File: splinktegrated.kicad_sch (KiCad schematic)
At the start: 65 parts, among them J1 USB_C_Receptacle_USB2.0, J10 NA_Ribbon, J11 NA_Serial, J12 NA_Conn_01x04_Female, J13 Conn_01x01_Socket, J14 Cirque, J15 Conn_01x01_Socket, J16 Conn_01x01_Socket, J17 Conn_01x01_Socket, J2 NA_Conn_01x04_Female, J3 NA_Conn_01x04_Female, J4 NA_Conn_01x04_Female, J5 Conn_01x02, J6 Cirque, J7 NA_trackball, J8 NA_Ribbon, J9 NA_RGB, SW1 NA_SW_SPST, SW2 NA_SW_SPST, U1 RP2040, U2 USBLC6-2P6, U3 XC6210B332MR-G, U4 USBLC6-2P6, U5 W25Q128JVS, Y1 Crystal_GND24

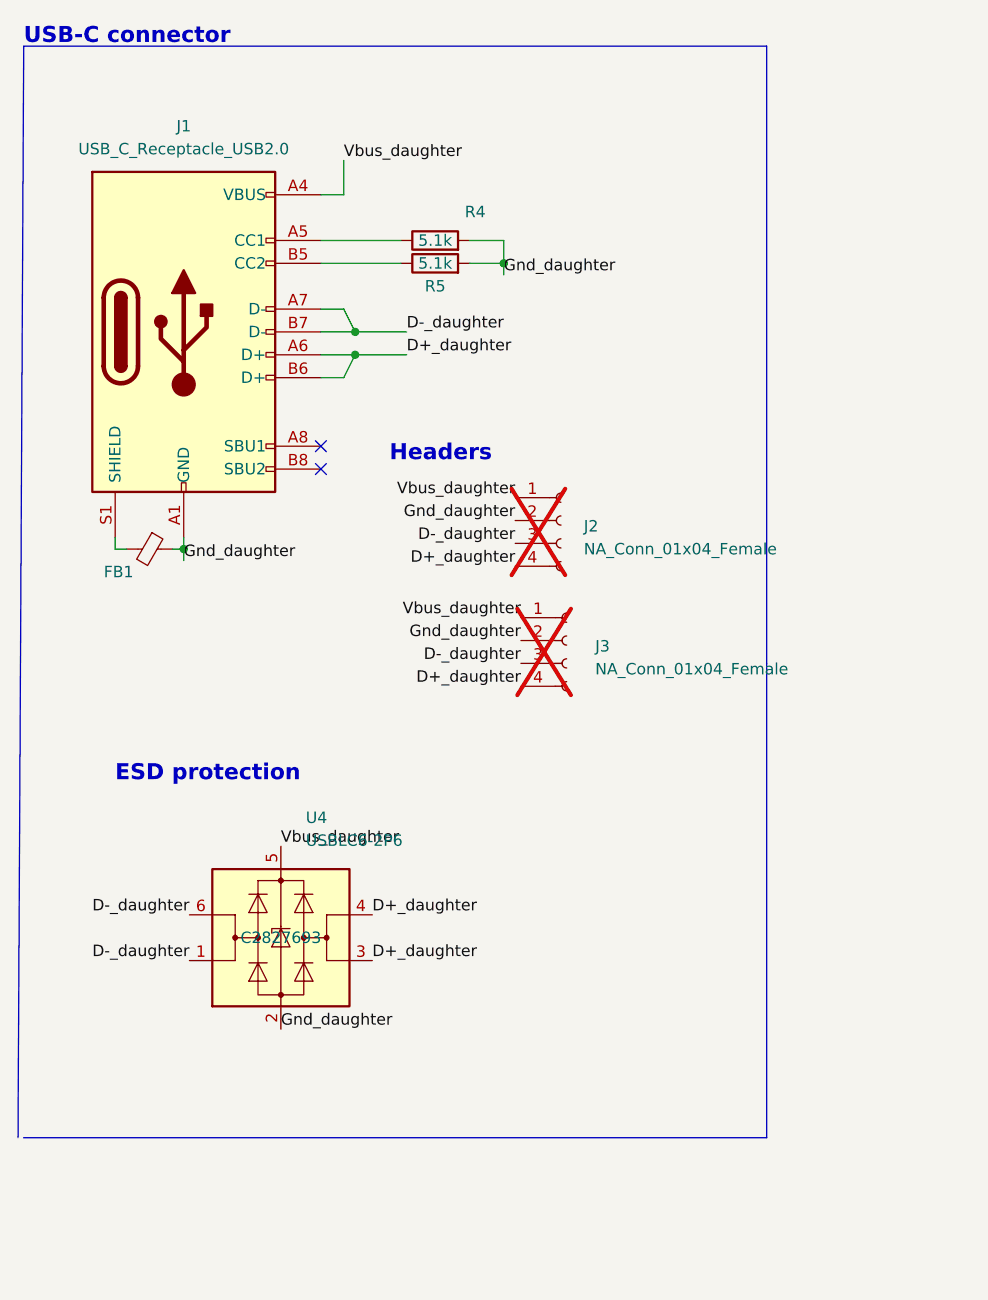
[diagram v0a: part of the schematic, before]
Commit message: schematic
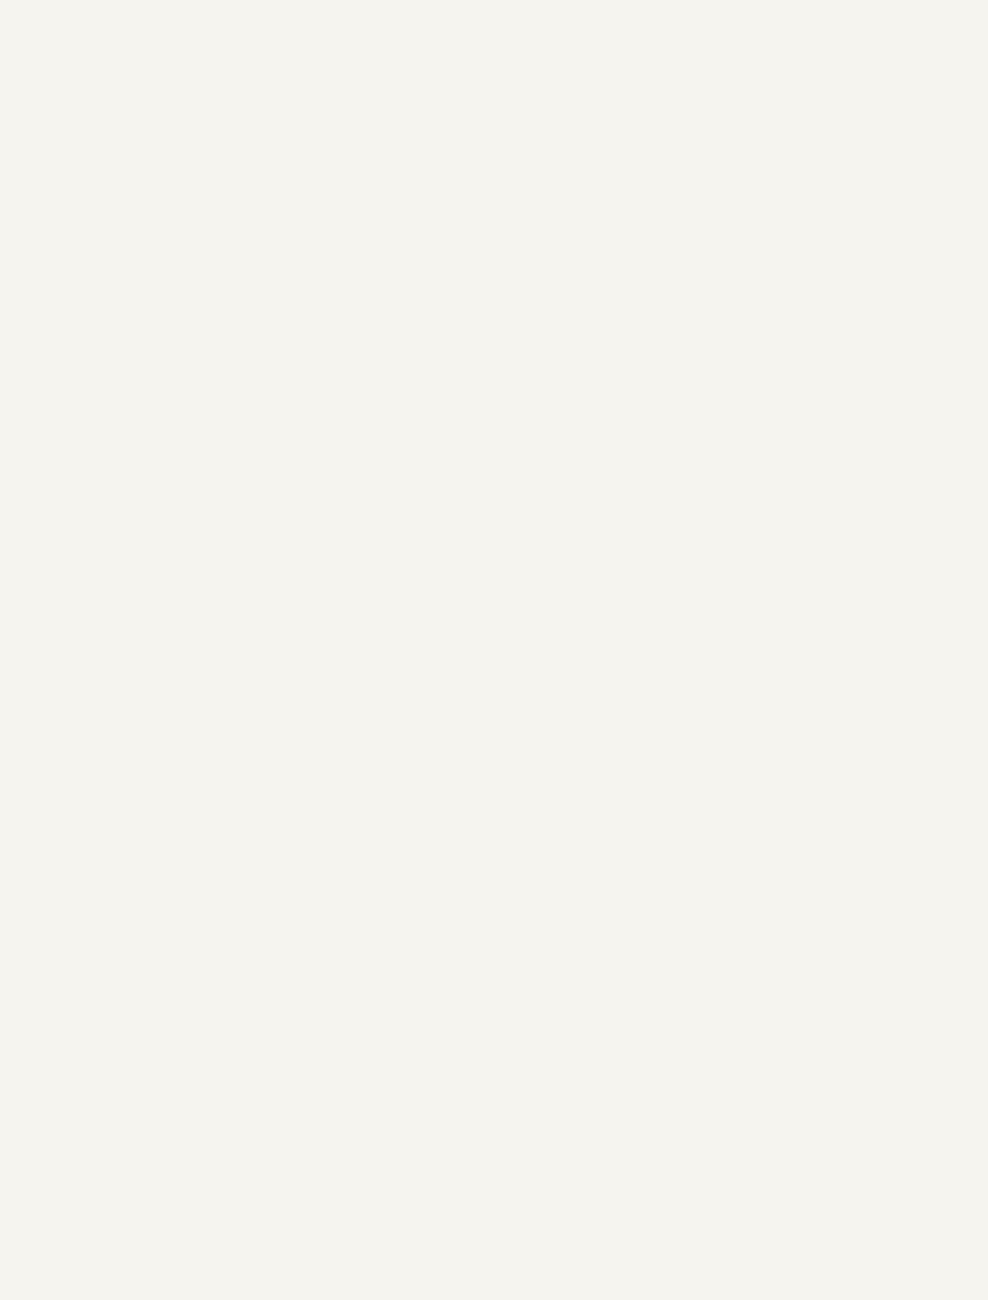
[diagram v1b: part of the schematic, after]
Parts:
- removed FB1: FerriteBead_Small, Inductor_SMD:L_0603_1608Metric, symbol Device:FerriteBead_Small
- removed J1: USB_C_Receptacle_USB2.0, drawings:GT-USB-7014C, symbol Connector:USB_C_Receptacle_USB2.0
- removed J2, J3: NA_Conn_01x04_Female, Library:PinHeader_1x04_P2.54mm_Vertical_USB, symbol Connector:Conn_01x04_Female
- removed R4, R5: 5.1k, Resistor_SMD:R_0402_1005Metric, symbol Device:R
- removed U4: USBLC6-2P6, Package_TO_SOT_SMD:SOT-666, symbol Power_Protection:USBLC6-2P6
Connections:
- no-connect marks 12 -> 10
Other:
- note removed: "ESD protection"
- note removed: "Headers"
- note removed: "USB-C connector"

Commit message: move to usb c serial
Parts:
- removed J11: NA_Serial, drawings:Jack_3.5mm_PJ320E_Horizontal_custom, symbol Connector:AudioJack4
- removed J12, J4: NA_Conn_01x04_Female, drawings:PinHeader_1x04_P2.54mm_Vertical, symbol Connector:Conn_01x04_Female
- removed NA_J6: Serial, drawings:Jack_3.5mm_PJ320E_Horizontal_custom, symbol Connector:AudioJack4
- removed NA_JP1, NA_JP2: NA_Jumper_2_Open, local-libraries:SolderJumper-2_P1.3mm_Open_RoundedPad1.0x1.5mm, symbol Jumper:Jumper_2_Open
- removed NA_JP8, NA_JP9: NA_Jumper_2_Open, local-libraries:SolderJumper-2_P1.3mm_Open_TrianglePad1.0x1.5mm, symbol Jumper:Jumper_2_Open
- added FB1, FB2: FerriteBead_Small, Inductor_SMD:L_0603_1608Metric, symbol Device:FerriteBead_Small
- added J1, J18: USB_C_Receptacle_USB2.0, drawings:GT-USB-7014C, symbol Connector:USB_C_Receptacle_USB2.0
- added R4, R5: 5.1k, Resistor_SMD:R_0402_1005Metric, symbol Device:R
- added U4: USBLC6-2P6, Package_TO_SOT_SMD:SOT-666, symbol Power_Protection:USBLC6-2P6
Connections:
- net +3V3: now also J18.A4 (VBUS), J18.A9 (VBUS), J18.B4 (VBUS), J18.B9 (VBUS)
- net D+: now also J1.A6 (D+), J1.B6 (D+), U4.3 (I/O2), U4.4 (I/O2)
- net D-: now also J1.A7 (D-), J1.B7 (D-), U4.1 (I/O1), U4.6 (I/O1)
- net GND: now also FB1.1, FB2.1, J1.A1 (GND), J1.A12 (GND), J1.B1 (GND), J1.B12 (GND), J18.A1 (GND), J18.A12 (GND), J18.B1 (GND), J18.B12 (GND), R4.2, R5.2, U4.2 (GND)
- net VBUS: now also J1.A4 (VBUS), J1.A9 (VBUS), J1.B4 (VBUS), J1.B9 (VBUS), U4.5 (VBUS)
- net serial_l: now also J18.A6 (D+), J18.B6 (D+)
- net serial_l2: now also J18.A7 (D-), J18.B7 (D-)
- new net: J1.A5 (CC1), R4.1
- new net: FB2.2, J18.S1 (SHIELD)
- new net: J1.B5 (CC2), R5.1
- new net: FB1.2, J1.S1 (SHIELD)
- no-connect marks 10 -> 16
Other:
- note added: "ESD protection"
- note added: "Headers"
- note added: "Serial connector"
- note added: "USB-C connector"
- moved on the sheet: D2, F1, U2

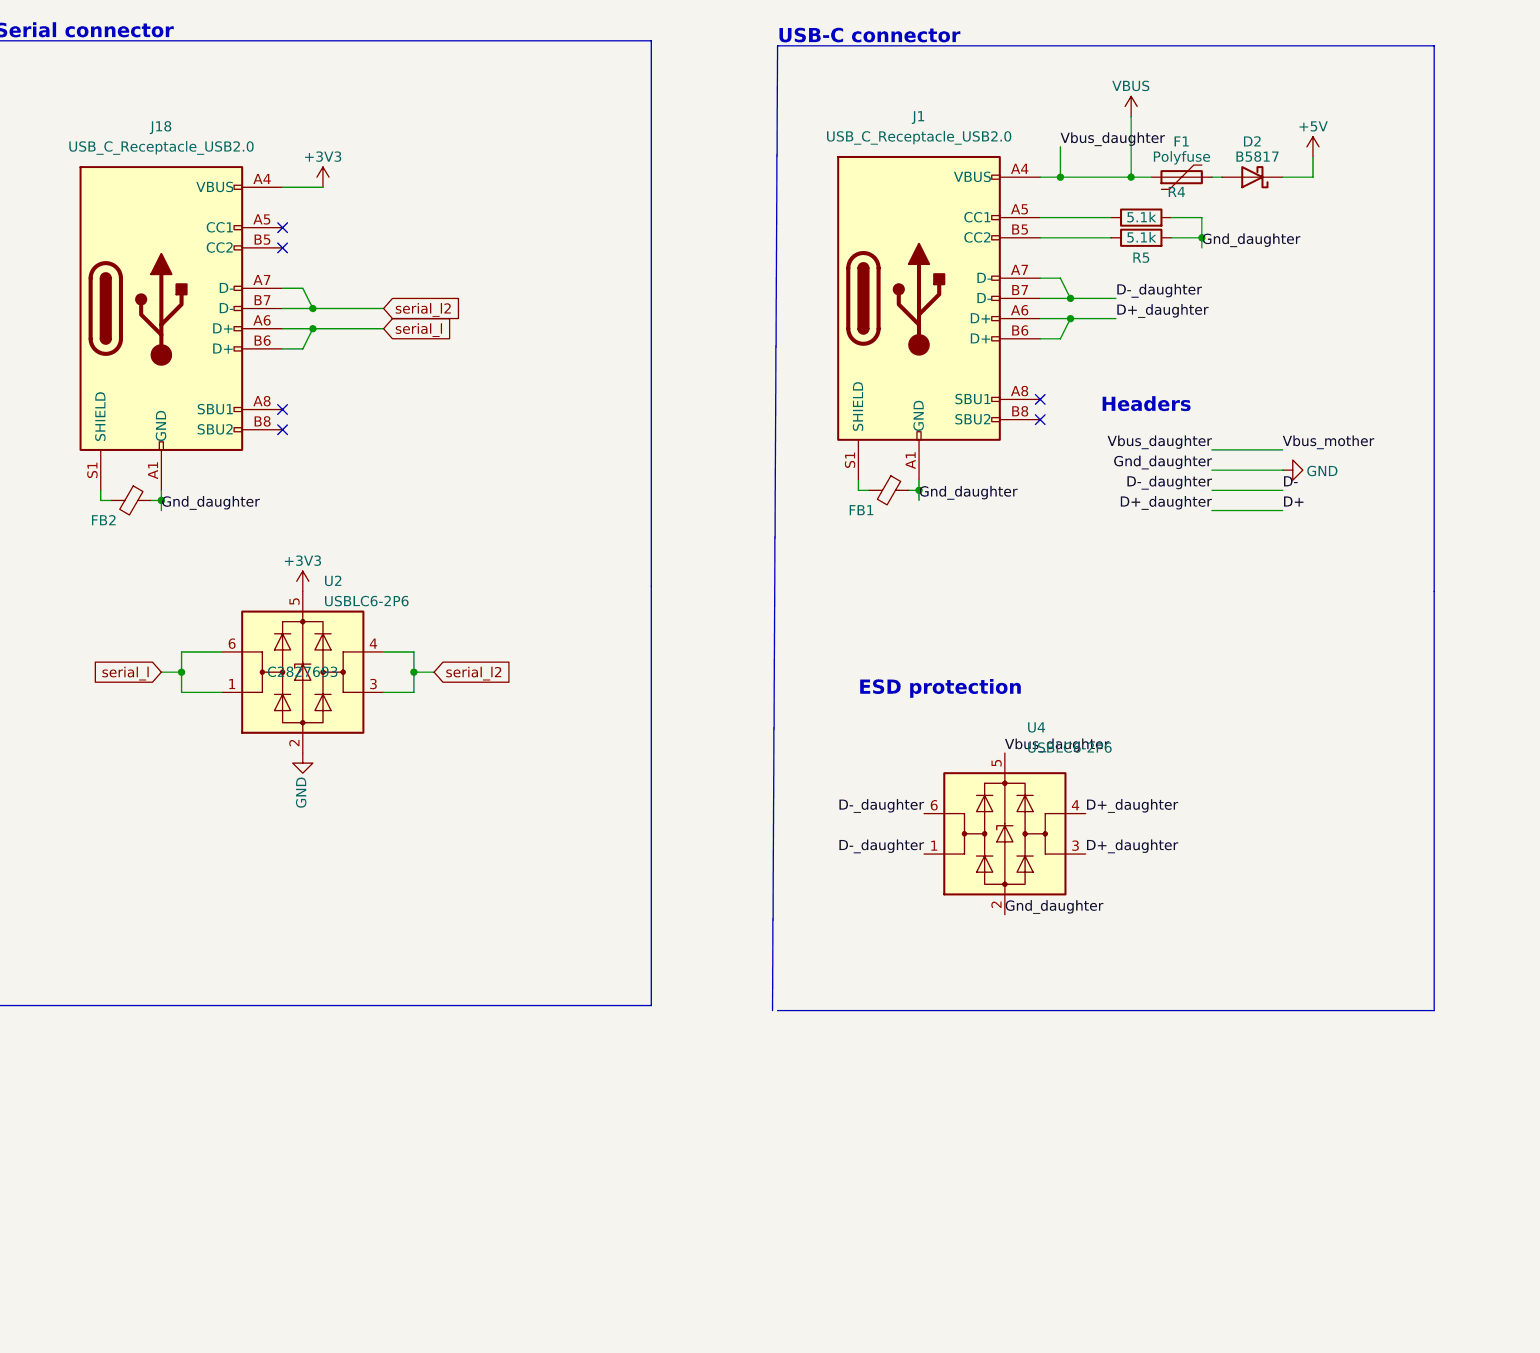
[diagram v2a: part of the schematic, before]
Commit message: 5V interconnect
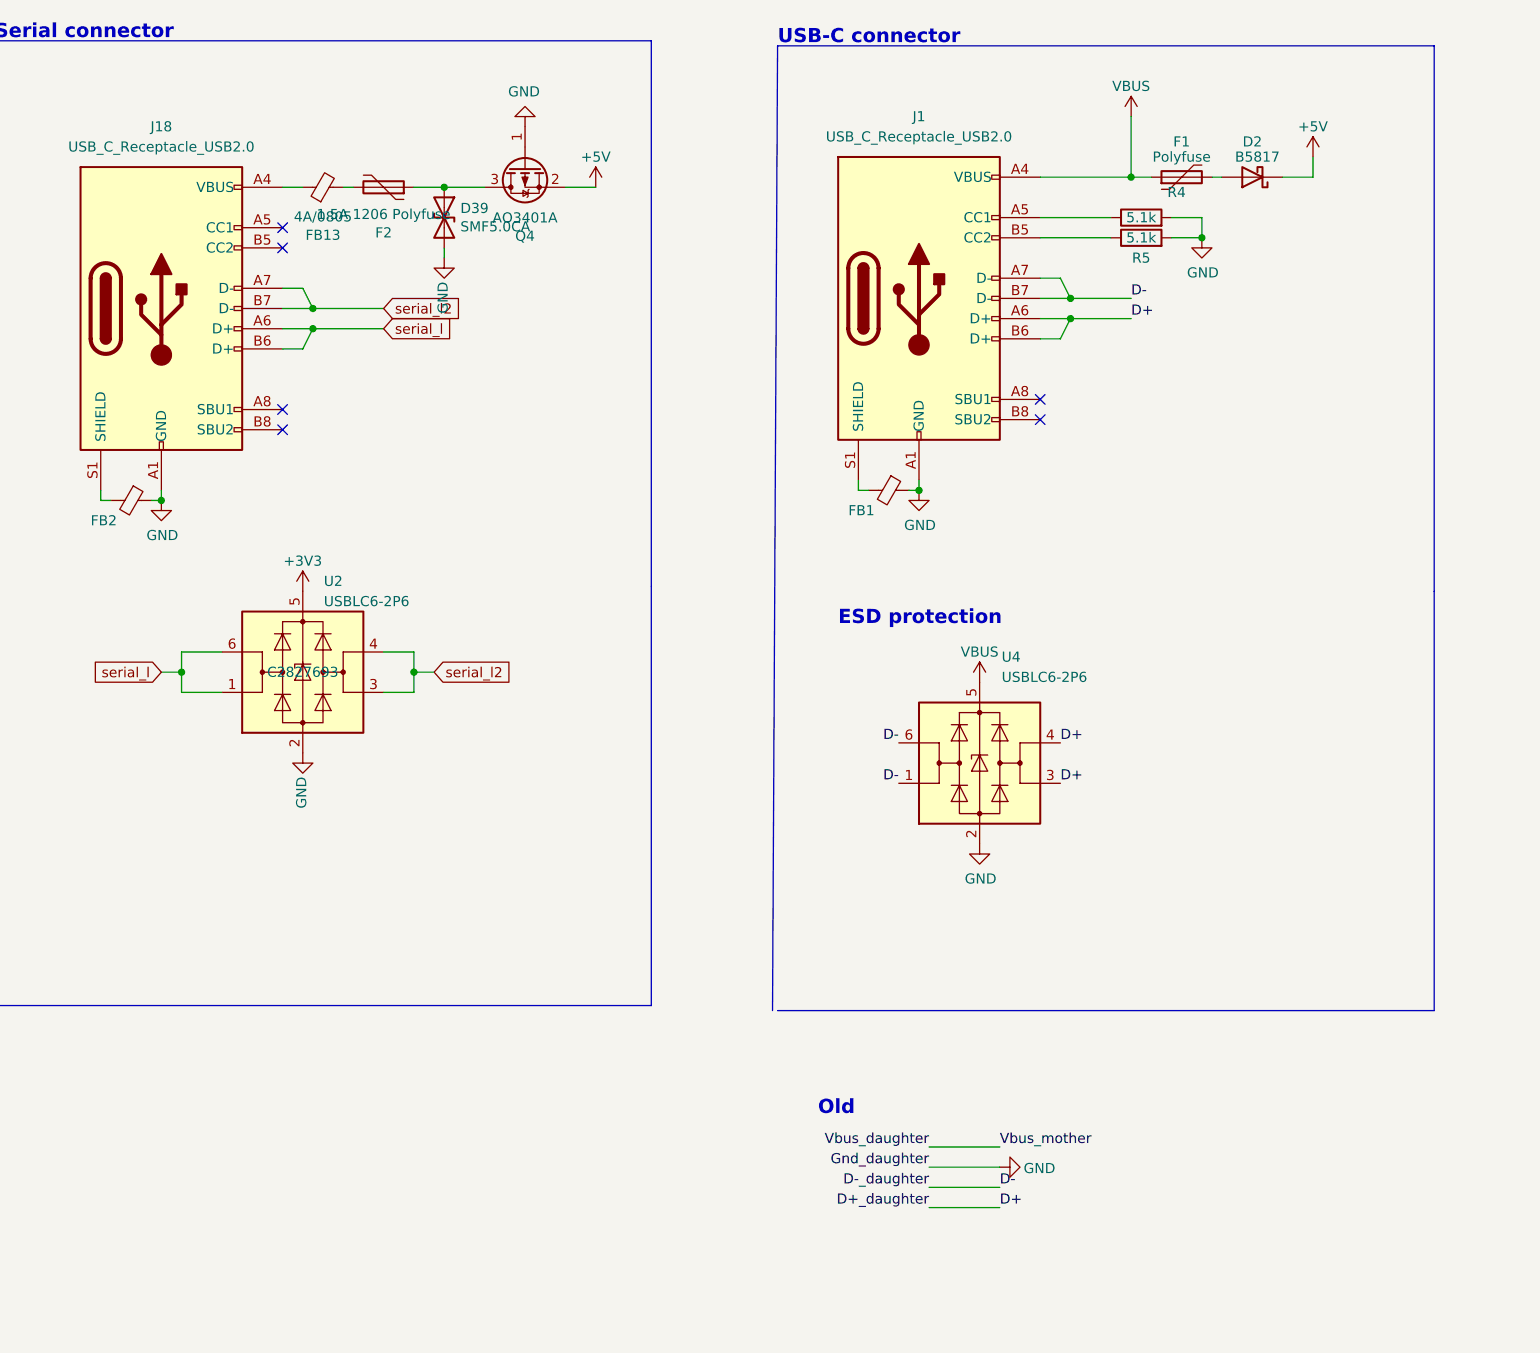
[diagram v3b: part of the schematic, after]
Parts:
- added D39: SMF5.0CA, reversible-kicad-footprints:D_SOD-123, symbol Device:D_TVS
- added F2: 1.5A 1206 Polyfuse, reversible-kicad-footprints:Fuse_1206_3216Metric, symbol Device:Polyfuse
- added FB13: 4A/0805, reversible-kicad-footprints:L-0805_2012Metric, symbol Device:Ferrite_Bead_Small
- added Q4: AO3401A, reversible-kicad-footprints:SOT-23-3, symbol Transistor_FET:AO3401A
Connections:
- net +3V3: no longer J18.A4 (VBUS), J18.A9 (VBUS), J18.B4 (VBUS), J18.B9 (VBUS)
- net +5V: now also Q4.2 (S)
- net GND: now also D39.2 (A2), Q4.1 (G)
- new net: D39.1 (A1), F2.1, Q4.3 (D)
- new net: F2.2, FB13.2
- new net: FB13.1, J18.A4 (VBUS), J18.A9 (VBUS), J18.B4 (VBUS), J18.B9 (VBUS)
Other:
- note added: "Old"
- note removed: "Headers"
- moved on the sheet: U4
